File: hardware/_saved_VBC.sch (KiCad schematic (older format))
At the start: 27 parts, among them J1 Jack-DC, J2 USB_OTG, J3 6P6C, J4 Conn_01x02, J5 RJ11, J6 RJ11, J7 RJ11, J8 RJ11, K1 RELAY_Metaltex, K2 RELAY_Metaltex, K3 RELAY_Metaltex, K4 RELAY_Metaltex, P1 CONN_01X01, Q1 BC817, Q2 BC817, Q3 BC817, Q4 BC817, U1 TS5A21366, U2 TS5A21366

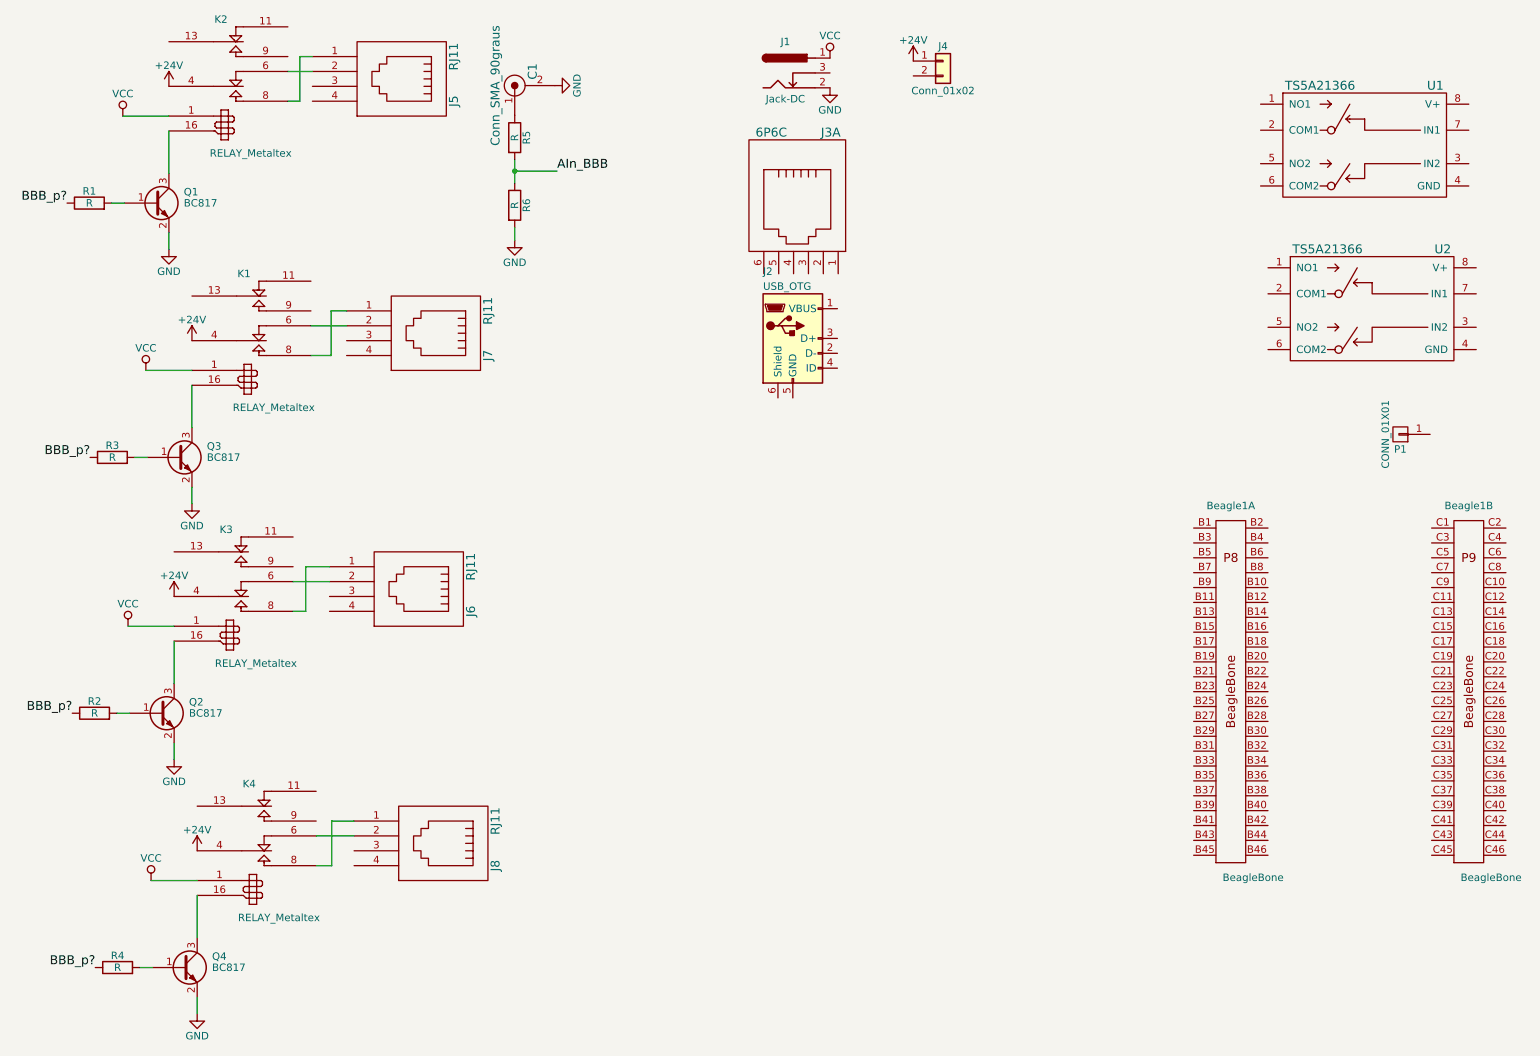
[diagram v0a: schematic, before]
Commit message: updated hardware files
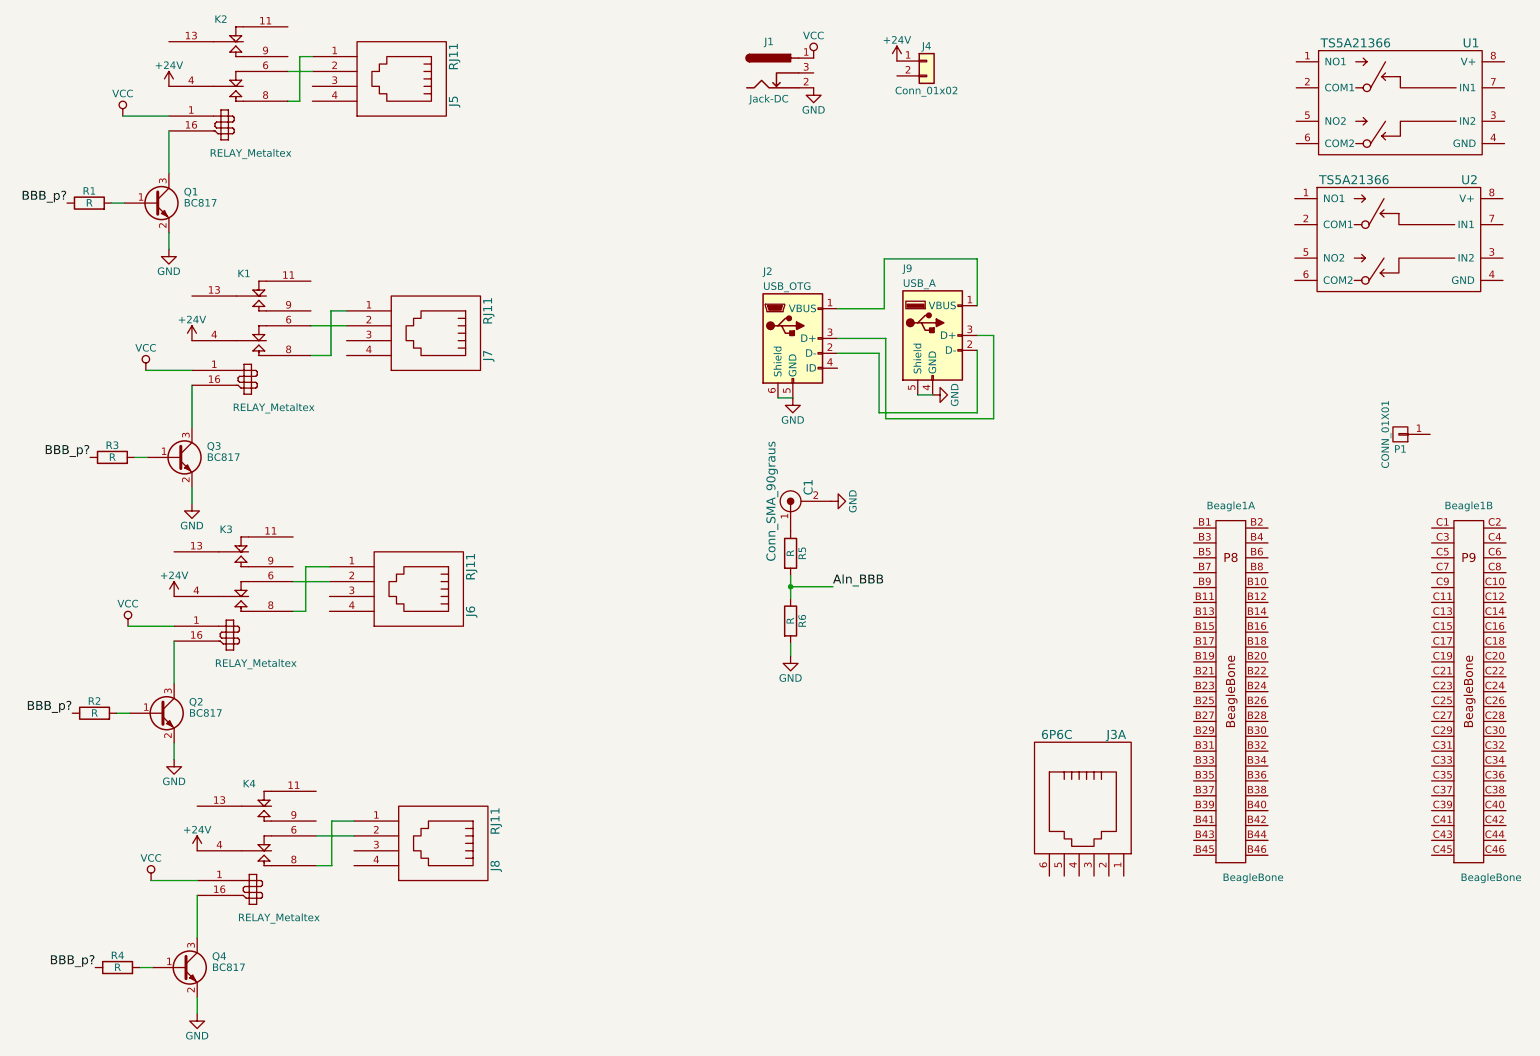
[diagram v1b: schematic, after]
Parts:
- added J9: USB_A, Connectors:USB_A, symbol USB_A
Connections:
- net GND: now also J2.5 (GND), J2.6 (Shield), J9.4 (GND), J9.5 (Shield)
- net at J2.1 (VBUS): now also J9.1 (VBUS)
- net at J2.2 (D-): now also J9.2 (D-)
- net at J2.3 (D+): now also J9.3 (D+)
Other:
- moved on the sheet: C1, J1, J3A, J4, R5, R6, U1, U2
